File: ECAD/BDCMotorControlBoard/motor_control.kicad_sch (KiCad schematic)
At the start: 24 parts, among them J1 Motor Connector, J4 Limit switch, J5 Limit switch, U10 PGA112, U2 DRV8870DDA, U3 INA180A1

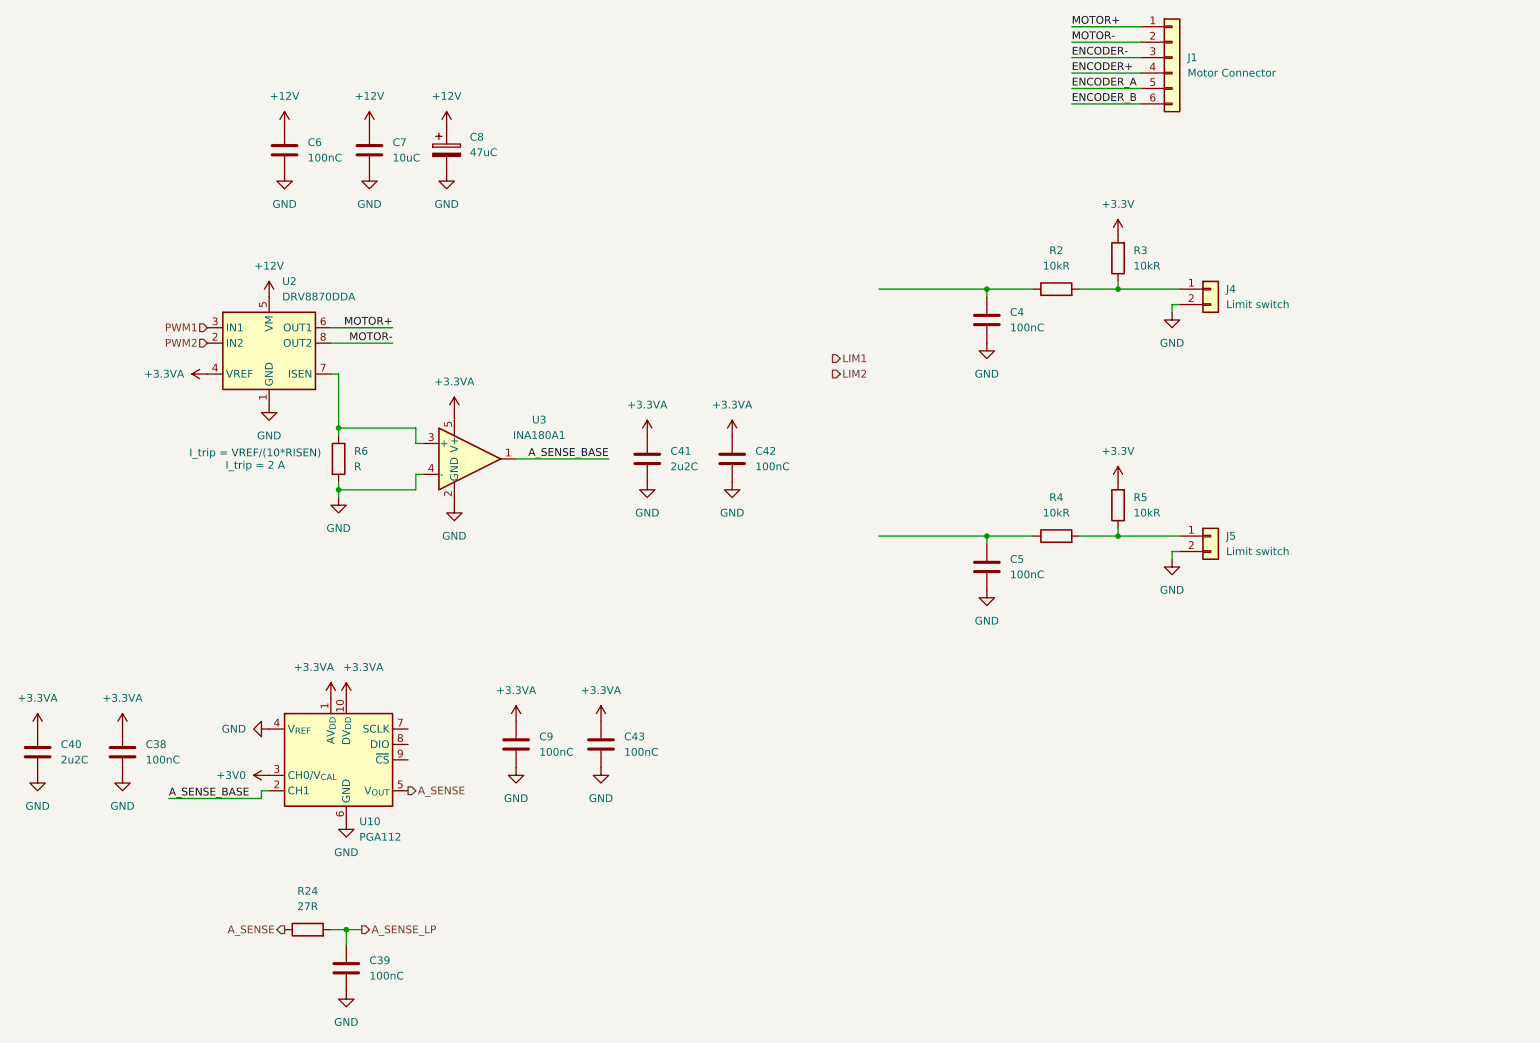
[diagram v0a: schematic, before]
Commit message: Progressed ECAD.
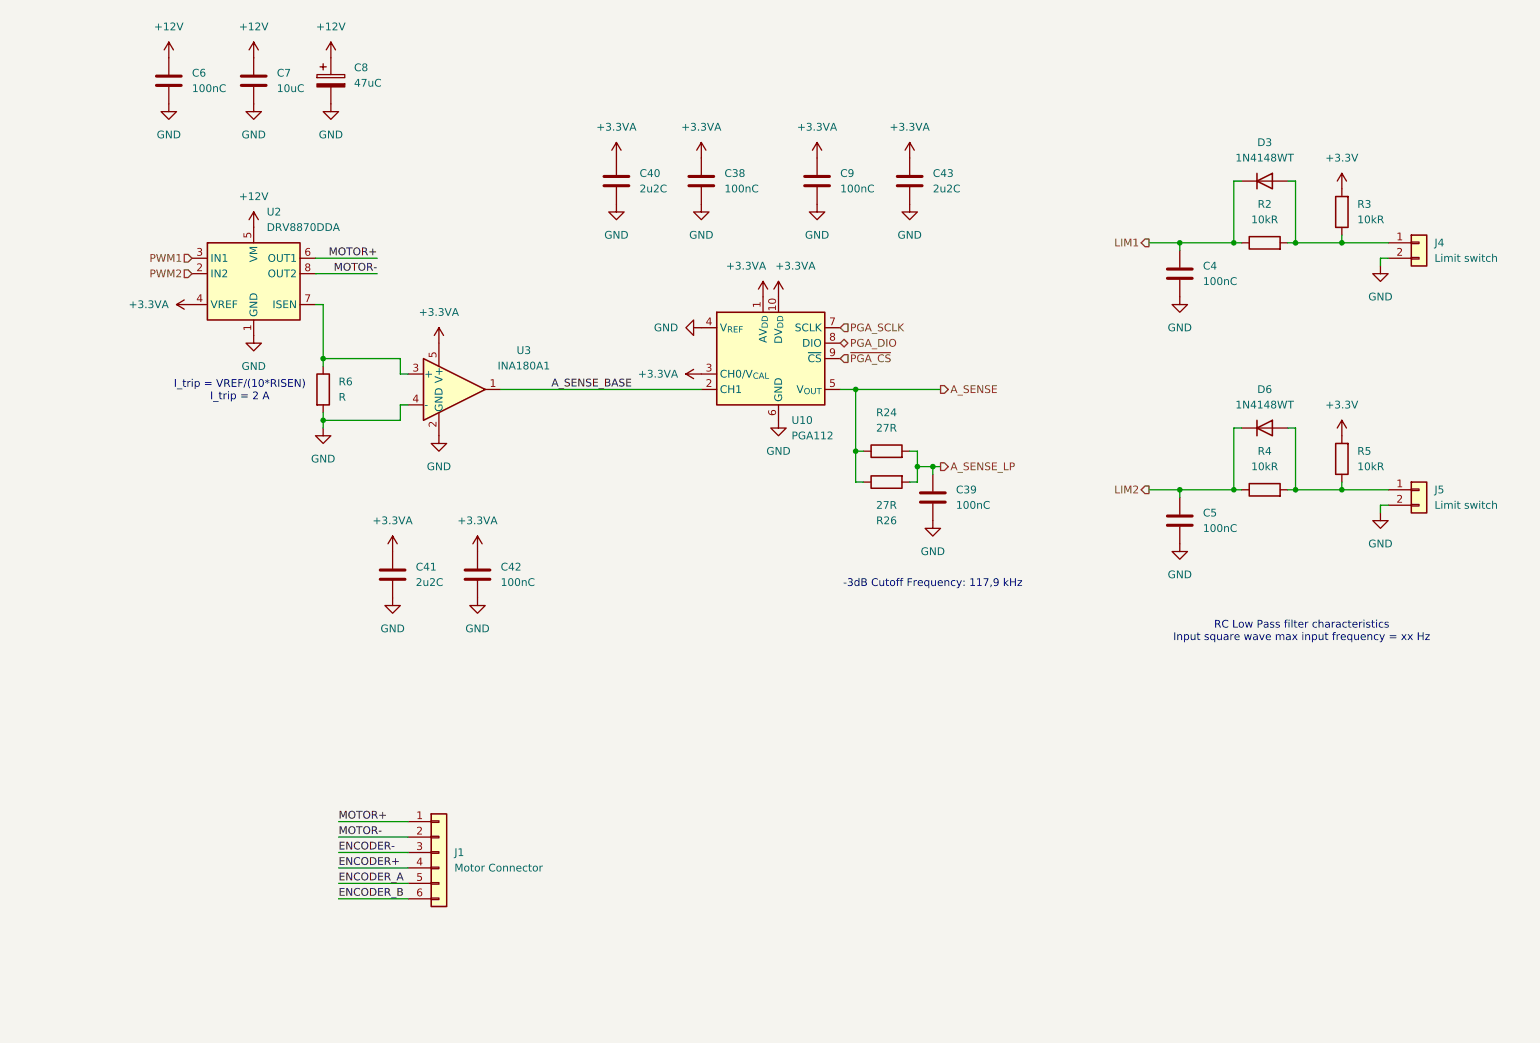
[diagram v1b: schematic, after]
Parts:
- added D3, D6: 1N4148WT, Diode_SMD:D_SOD-523, symbol Diode:1N4148WT
- added R26: 27R, symbol Device:R
- C43: value 100nC -> 2u2C; footprint Capacitor_SMD:C_0805_2012Metric -> Capacitor_SMD:C_0402_1005Metric; MPN (none) -> GRM155R60J225ME01D
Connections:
- net +3V0 is gone; now on net +3.3VA: U10.3 (CH0/V_{CAL})
- net A_SENSE: now also R26.1
- net A_SENSE_LP: now also R26.2
- net LIM1: now also C4.1, R2.1, D3.1 (K)
- net LIM2: now also C5.1, R4.1, D6.1 (K)
- net at J4.1 (Pin_1), R2.2, R3.1: now also D3.2 (A)
- net PGA_SCLK: now reaches U10.7 (SCLK)
- net PGA_DIO: now reaches U10.8 (DIO)
- net ~{PGA_CS}: now reaches U10.9 (~{CS})
- net at J5.1 (Pin_1), R4.2, R5.1: now also D6.2 (A)
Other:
- note added: "-3dB Cutoff Frequency: 117,9 kHz"
- note added: "RC Low Pass filter characteristics Input square wave max input frequency = xx Hz"
- moved on the sheet: C38, C39, C4, C40, C41, C42, C5, C6, C7, C8, C9, J1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
